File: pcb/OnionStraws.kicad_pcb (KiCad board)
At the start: 2 copper layers, 100 x 50 mm, 61 parts, among them J1 Conn_01x04, J2 8P8C, Q1 Si2309CDS, Q2 Si2309CDS, SW1 SW_Push, U1 74LVC2G07, U2 74LVC2G07_3v3, U3 ESP32, U4 APX803L

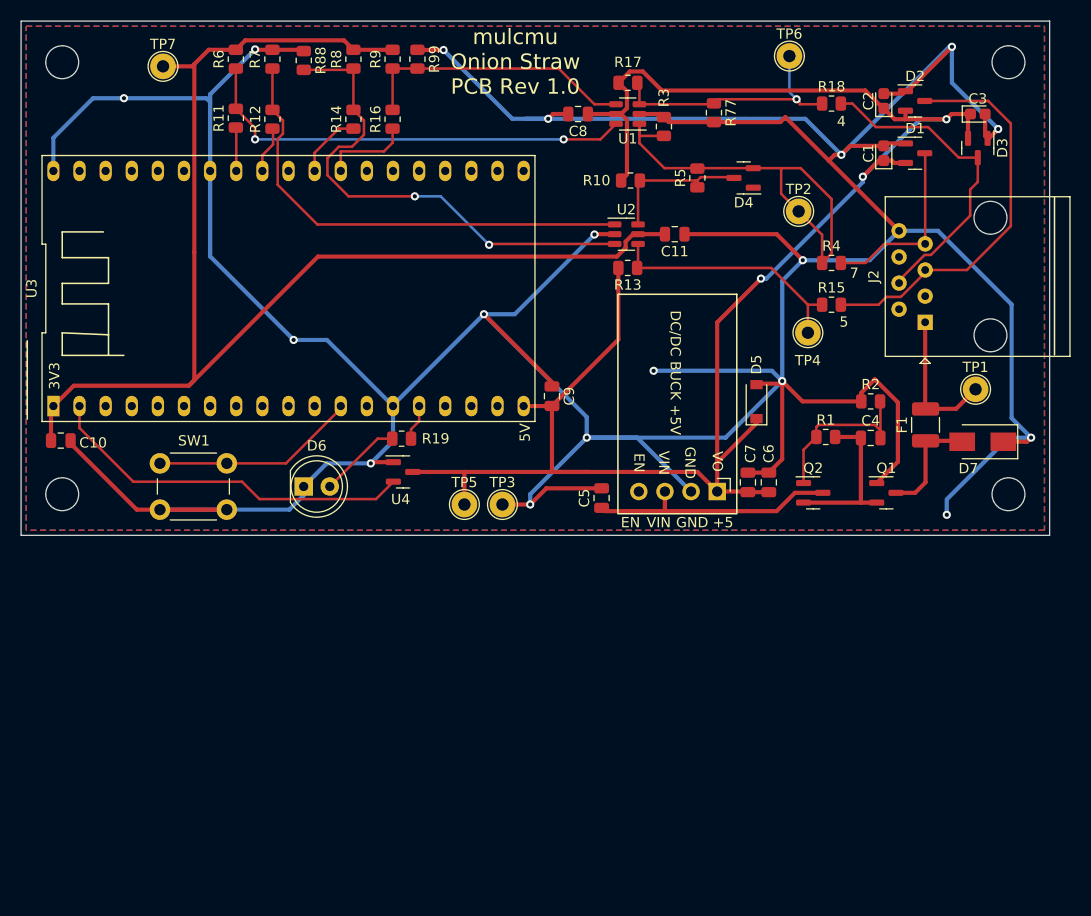
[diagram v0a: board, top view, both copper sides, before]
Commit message: v2 beta
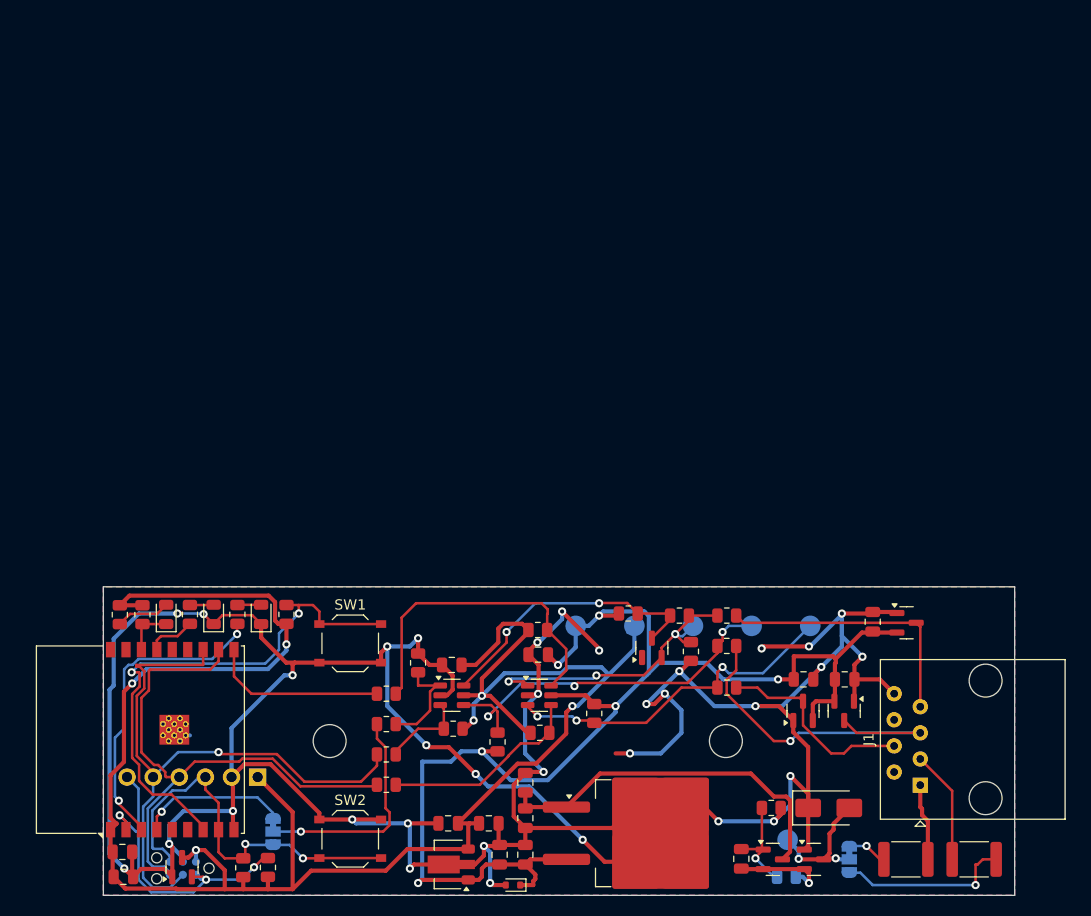
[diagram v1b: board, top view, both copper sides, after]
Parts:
- removed H3, H4: MountingHole, MountingHole:MountingHole_3.2mm_M3_DIN965
- removed R77: 270k, Resistor_SMD:R_0805_2012Metric
- removed R88, R99: 10K, Resistor_SMD:R_0805_2012Metric
- removed TP3, TP7: TestPoint, TestPoint:TestPoint_THTPad_D2.5mm_Drill1.2mm
- added C12: 100n, Capacitor_SMD:C_0805_2012Metric, F.Cu at (81.5, 106.0)
- added C13: 10u, Capacitor_SMD:C_0805_2012Metric, F.Cu at (80.5, 103.0)
- added C14: 100n, Capacitor_SMD:C_0805_2012Metric, F.Cu at (76.5, 103.0)
- added D8: 5.2V, Diode_SMD:D_SOD-523, F.Cu at (82.8, 109.0)
- added D9: BAV99, Package_TO_SOT_SMD:SOT-23, F.Cu at (96.3, 85.9)
- added F2: Polyfuse, Fuse:Fuse_1812_4532Metric, F.Cu at (121.0, 106.5)
- added INPUT POWER: TestPoint, TestPoint:TestPoint_Pad_D2.0mm, B.Cu at (109.5, 104.6)
- added J3: TC2030, Connector:Tag-Connect_TC2030-IDC-NL_2x03_P1.27mm_Vertical, B.Cu at (50.7, 107.4)
- added JP1: FirstBuild, Jumper:SolderJumper-3_P1.3mm_Bridged12_RoundedPad1.0x1.5mm_NumberLabels, B.Cu at (59.5, 103.8)
- added Power Pin: AltPwr, Jumper:SolderJumper-3_P1.3mm_Bridged12_RoundedPad1.0x1.5mm_NumberLabels, B.Cu at (115.5, 106.5)
- added R20: 10K, Resistor_SMD:R_0805_2012Metric, F.Cu at (81.3, 95.1)
- added R21: 220k, Resistor_SMD:R_0805_2012Metric, F.Cu at (90.7, 92.3)
- added R22: 4K7, Resistor_SMD:R_0805_2012Metric, F.Cu at (99.0, 82.8)
- added R23: 1K, Resistor_SMD:R_0805_2012Metric, F.Cu at (103.6, 82.8)
- added R24: 1K, Resistor_SMD:R_0805_2012Metric, F.Cu at (103.6, 85.8)
- added R25: 1K, Resistor_SMD:R_0805_2012Metric, F.Cu at (103.6, 89.8)
- added SW2: SW_Push, Button_Switch_SMD:SW_Push_1P1T_XKB_TS-1187A, F.Cu at (67.0, 104.5)
- added U5: 74LVC2G07_3v3, Package_TO_SOT_SMD:SOT-23-6, F.Cu at (76.9, 90.5)
- added U6: AP2205-3.3, Package_TO_SOT_SMD:SOT-89-3, F.Cu at (76.5, 107.0)
- C1, C3: footprint Capacitor_Tantalum_SMD:CP_EIA-1608-10_AVX-L -> Capacitor_SMD:C_0805_2012Metric
- C10, C5, C6: value 10u -> 100n
- C11, C9: value 100n -> 10u
- C2: value 100n -> 1u; footprint Capacitor_Tantalum_SMD:CP_EIA-1608-10_AVX-L -> Capacitor_SMD:C_0805_2012Metric
- C4, C7: value 1u -> 100n
- C8: value 100n -> 1u
- D4: value BAV99 -> GRN; footprint Package_TO_SOT_SMD:SOT-23 -> LED_SMD:LED_0805_2012Metric
- D5: value 5.2V -> RED; footprint Diode_SMD:D_SOD-123 -> LED_SMD:LED_0805_2012Metric
- D6: value LED -> YLW; footprint LED_THT:LED_D5.0mm -> LED_SMD:LED_0805_2012Metric
- F1: footprint Resistor_SMD:R_1210_3225Metric_Pad1.30x2.65mm_HandSolder -> Fuse:Fuse_1812_4532Metric
- J1: value Conn_01x04 -> 8P8C; footprint Connector_PinHeader_2.54mm:PinHeader_1x04_P2.54mm_Horizontal -> Connector_RJ:RJ45_Amphenol_54602-x08_Horizontal
- J2: value 8P8C -> 1x6; footprint Connector_RJ:RJ45_Amphenol_54602-x08_Horizontal -> Connector_PinHeader_2.54mm:PinHeader_1x06_P2.54mm_Vertical; moved to B.Cu
- R1: value DNP -> 10K
- R10, R13: value 10K -> 1K
- R14, R15, R16: value 1K -> 10K
- R17, R3: value 270k -> 10K
- R18: value 1K -> 220k
- R19: value 220 -> 10K
- R2: value 1M -> 10K
- R4: value 1K -> 220
- R5: value 4K7 -> 10K
- R6, R7: value 10K -> 220
- R8: value 10K -> DNP; moved to B.Cu
- R9: value 10K -> 1M
- SW1: footprint Button_Switch_THT:SW_PUSH_6mm_H13mm -> Button_Switch_SMD:SW_Push_1P1T_XKB_TS-1187A
- TP1, TP2, TP4, TP5, TP6: footprint TestPoint:TestPoint_THTPad_D2.5mm_Drill1.2mm -> TestPoint:TestPoint_Pad_D2.0mm; moved to B.Cu
- U1: value 74LVC2G07 -> APX803L20-29SA-7; footprint Package_TO_SOT_SMD:SOT-23-6 -> Package_TO_SOT_SMD:SOT-23
- U2: value 74LVC2G07_3v3 -> ESP32-C3-WROOM-02; footprint Package_TO_SOT_SMD:SOT-23-6 -> RF_Module:ESP32-C3-WROOM-02
- U3: value ESP32 -> L7805; footprint Library:DIP-38_900_ELL -> Package_TO_SOT_SMD:TO-263-2
- U4: value APX803L -> 74LVC2G07; footprint Package_TO_SOT_SMD:SOT-23 -> Package_TO_SOT_SMD:SOT-23-6
- moved C2 104.0 mm to (44.9, 105.8), turned to 0 degrees
- moved R8 90.0 mm to (109.4, 108.2), turned to 0 degrees
- moved U1 85.1 mm to (50.6, 107.3), turned to 90 degrees
- moved C4 84.3 mm to (45.0, 108.2), turned to 180 degrees
- moved R3 81.7 mm to (59.0, 107.3), turned to -90 degrees
- moved R9 81.6 mm to (107.9, 101.5), turned to 180 degrees
- moved J2 78.5 mm to (58.0, 98.5)
- moved R4 77.2 mm to (44.6, 82.7), turned to 90 degrees
- moved R2 76.0 mm to (56.6, 107.3), turned to 90 degrees
- moved C8 74.1 mm to (105.0, 106.5), turned to 90 degrees
- moved H1 70.9 mm to (65.0, 95.0)
- moved H2 68.8 mm to (103.5, 95.0)
- moved R5 68.7 mm to (46.8, 82.7)
- moved D4 66.8 mm to (53.7, 82.7), turned to 90 degrees
- moved U2 66.1 mm to (49.7, 94.9), turned to 90 degrees
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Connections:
- C10 pad 1: +3V3 -> GND
- C10 pad 2: GND -> /p3
- C11 pad 1: GND -> +5V
- C11 pad 2: +3V3 -> GND
- C2 pad 1: +5V -> +3V3
- C4 pad 1: /p2 -> GND
- C4 pad 2: Net-(C4-Pad2) -> +3V3
- C5 pad 1: /p3 -> +5V
- C6 pad 1: +5V -> GND
- C6 pad 2: GND -> +3V3
- C8 pad 1: +5V -> /p2
- C8 pad 2: GND -> Net-(Q2-G)
- C9 pad 1: GND -> /p3
- C9 pad 2: +5V -> GND
- D4 pad 1: unconnected-(D4-Pad1) -> GND
- D4 pad 2: Net-(D4-Pad2) -> Net-(D4-A)
- D5 pad 1: +5V -> /DBG_LED
- D5 pad 2: GND -> Net-(D5-A)
- D6 pad 2: Net-(D6-Pad2) -> Net-(D6-A)
- F1 pad 1: /p1 -> /ALT_PWR
- F1 pad 2: VDC -> Net-(JP2-B)
- J1 pad 1: +5V -> VDC
- J1 pad 2: GND -> unconnected-(J1-Pad2)
- J1 pad 3: /p3 -> /ALT_PWR
- J1 pad 4: unconnected-(J1-Pad4) -> GEA_FullTx
- J2 pad 1: VDC -> +3V3
- J2 pad 2: unconnected-(J2-Pad2) -> GND
- J2 pad 3: unconnected-(J2-Pad3) -> /BOOT
- J2 pad 4: GEA_FullTx -> GEA3_TX
- J2 pad 5: GEA_FullRx -> GEA3_RX
- J2 pad 6: unconnected-(J2-Pad6) -> /EN
- Q2 pad 1: Net-(C4-Pad2) -> Net-(Q2-G)
- R1 pad 1: Net-(C4-Pad2) -> /BOOT_SEL
- R1 pad 2: /p2 -> +3V3
- R10 pad 1: Net-(D4-Pad3) -> GEA2_RX
- R10 pad 2: +5V -> Net-(R10-Pad2)
- R11 pad 1: Net-(R11-Pad1) -> GEA2_TX
- R12 pad 1: Net-(R12-Pad1) -> GEA3_RX
- R13 pad 1: Net-(R13-Pad1) -> GEA3_TX
- R13 pad 2: +5V -> Net-(R13-Pad2)
- R14 pad 1: Net-(R14-Pad1) -> Net-(R10-Pad2)
- R14 pad 2: Net-(R14-Pad2) -> +3V3
- R15 pad 1: Net-(R13-Pad1) -> GND
- R15 pad 2: GEA_FullRx -> Net-(R11-Pad2)
- R16 pad 1: Net-(R16-Pad1) -> Net-(R12-Pad2)
- R16 pad 2: Net-(R16-Pad2) -> +3V3
- R17 pad 1: Net-(R17-Pad1) -> Net-(R13-Pad2)
- R17 pad 2: +5V -> +3V3
- R18 pad 1: Net-(R17-Pad1) -> Net-(D9-A)
- R18 pad 2: GEA_FullTx -> GND
- R19 pad 1: Net-(D6-Pad2) -> Net-(D9-K-Pad3)
- R19 pad 2: Net-(R19-Pad2) -> +5V
- R2 pad 1: GND -> +3V3
- R2 pad 2: Net-(C4-Pad2) -> /BOOT
- R3 pad 1: Net-(D4-Pad2) -> /EN
- R3 pad 2: GND -> +3V3
- R4 pad 1: Net-(D4-Pad2) -> Net-(D5-A)
- R4 pad 2: GEA_HalfDplx -> +3V3
- R5 pad 1: Net-(D4-Pad3) -> /DBG_LED
- R5 pad 2: Net-(D4-Pad2) -> +3V3
- R6 pad 1: Net-(R11-Pad2) -> /LED2
- R6 pad 2: +3V3 -> Net-(D4-A)
- R7 pad 1: GND -> Net-(D6-A)
- R7 pad 2: Net-(R12-Pad2) -> /LED1
- R8 pad 1: Net-(R14-Pad2) -> Net-(Q2-G)
- R8 pad 2: +3V3 -> /p2
- R9 pad 1: Net-(R16-Pad2) -> GND
- R9 pad 2: +3V3 -> Net-(Q2-G)
- SW1 pad 1: GND -> /BOOT_SEL
- SW1 pad 2: Net-(SW1-Pad2) -> GND
- TP1 pad 1: VDC -> +5V
- TP2 pad 1: Net-(D4-Pad2) -> +3V3
- TP4 pad 1: Net-(R13-Pad1) -> Net-(D9-A)
- TP5 pad 1: +5V -> Net-(R20-Pad1)
- TP6 pad 1: Net-(R17-Pad1) -> Net-(R21-Pad1)
- U1 pad 1: Net-(D4-Pad2) -> GND
- U1 pad 2: GND -> /EN
- U1 pad 3: Net-(R17-Pad1) -> +3V3
- U2 pad 1: Net-(R12-Pad2) -> +3V3
- U2 pad 2: GND -> /EN
- U2 pad 3: Net-(R14-Pad2) -> /LED1
- U2 pad 4: Net-(R13-Pad1) -> Net-(JP1-A)
- U2 pad 5: +3V3 -> unconnected-(U2-IO6-Pad5)
- U2 pad 6: Net-(D4-Pad3) -> unconnected-(U2-IO7-Pad6)
- U3 pad 1: +3V3 -> /p3
- U3 pad 2: Net-(U3-Pad2) -> GND
- U3 pad 3: unconnected-(U3-Pad3) -> +5V
- U4 pad 1: GND -> Net-(D9-A)
- U4 pad 2: Net-(U3-Pad2) -> GND
- U4 pad 3: +5V -> Net-(R21-Pad1)
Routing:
- net GND: track 481.7 -> 358.9 mm, vias 18 -> 34
- net +3V3: track 125.4 -> 196.2 mm, vias 0 -> 6
- net GEA3_RX: track 0.00 -> 61.0 mm, vias 0 -> 1
- net GEA3_TX: track 0.00 -> 54.9 mm
- net +5V: track 179.2 -> 126.3 mm, vias 3 -> 6
- net /BOOT_SEL: track 0.00 -> 51.3 mm, vias 0 -> 2
- net Net-(R14-Pad2): track 48.6 -> 0.00 mm, vias 2 -> 0
- net Net-(D4-Pad2): track 43.8 -> 0.00 mm
- net /BOOT: track 0.00 -> 38.4 mm, vias 0 -> 2
- net Net-(R12-Pad2): track 46.3 -> 8.35 mm
- net Net-(R20-Pad1): track 0.00 -> 37.0 mm, vias 0 -> 3
- net Net-(U3-Pad2): track 36.2 -> 0.00 mm
- net Net-(R21-Pad1): track 0.00 -> 33.6 mm, vias 0 -> 3
- net Net-(R11-Pad2): track 43.4 -> 10.4 mm, vias 2 -> 0
- net /EN: track 0.00 -> 31.9 mm, vias 0 -> 3
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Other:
- board size 100 x 50 mm -> 88.6 x 30 mm
- board text added: "3v3 GND BOOT EN RX TX"
- board text added: "5V 3v3 Half (7) Full RX (5) Full TX (4)"
- board text added: "DIY Wi-fi adapter for GEA2 and GEA3 Connect to appliance at your own risk!"
- board text added: "EN RX TX BOOT GND 3v3"
- board text added: "mulcmu Onion Straws Revision 2.0"
- board text removed: "+5"
- board text removed: "3V3"
- board text removed: "4"
- board text removed: "5"
- board text removed: "5V"
- board text removed: "7"
- board text removed: "EN"
- board text removed: "GND"
- board text removed: "VIN"
- board text removed: "mulcmu Onion Straw PCB Rev 1.0"
